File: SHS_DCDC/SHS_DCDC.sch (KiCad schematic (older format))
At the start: 16 parts, among them J1 Barrel_Jack, Q1 BSS84, U1 A0Z1283

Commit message: esp32 s2 mini placed
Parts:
- C1, C2, C3, C4, C5: symbol Device:C -> SHS_DCDC:C-Device
- J1: symbol Connector:Barrel_Jack -> SHS_DCDC:Barrel_Jack-Connector
- L1: symbol Device:L -> SHS_DCDC:L-Device
- Q1: symbol Transistor_FET:BSS84 -> SHS_DCDC:BSS84-Transistor_FET
- R1, R2, R3, R4, R5, R6, R7: symbol Device:R -> SHS_DCDC:R-Device
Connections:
- net labels added: GND-power
- net labels removed: GND
- wire segments 44 -> 42
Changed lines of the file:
@@
 $EndDescr
 $Comp
-L Device:R R1
+L SHS_DCDC:R-Device R1
 U 1 1 603C1DE3
 P 3450 1300
@@
 EN
 $Comp
-L power:GND #PWR0101
+L SHS_DCDC:GND-power #PWR0101
 U 1 1 603DA7E8
 P 4700 2100
 F 0 "#PWR0101" H 4700 1850 50  0001 C CNN
-F 1 "GND" H 4705 1927 50  0000 C CNN
+F 1 "GND-power" H 4705 1927 50  0000 C CNN
 F 2 "" H 4700 2100 50  0001 C CNN
 F 3 "" H 4700 2100 50  0001 C CNN
@@
 	4700 2100 4700 1800
 $Comp
-L Device:C C1
+L SHS_DCDC:C-Device C1
 U 1 1 603DBEB8
 P 5750 1150
@@
 	5150 1150 5600 1150
 $Comp
-L power:GND #PWR0102
+L SHS_DCDC:GND-power #PWR0102
 U 1 1 603DC622
 P 6100 1150
 F 0 "#PWR0102" H 6100 900 50  0001 C CNN
-F 1 "GND" V 6105 1022 50  0000 R CNN
+F 1 "GND-power" V 6105 1022 50  0000 R CNN
 F 2 "" H 6100 1150 50  0001 C CNN
 F 3 "" H 6100 1150 50  0001 C CNN
@@
 	6050 1850 6350 1850
 $Comp
-L Device:C C2
+L SHS_DCDC:C-Device C2
 U 1 1 603EC5C6
 P 6050 1600
@@
 $EndComp
 $Comp
-L Device:L L1
+L SHS_DCDC:L-Device L1
 U 1 1 603ED963
 P 6500 1850
@@
 	6850 3000 6850 3150
 $Comp
-L Device:R R2
+L SHS_DCDC:R-Device R2
 U 1 1 603C2934
 P 3850 1650
@@
 $EndComp
 $Comp
-L Device:R R3
+L SHS_DCDC:R-Device R3
 U 1 1 603EF351
 P 6850 2150
@@
 $EndComp
 $Comp
-L Device:R R4
+L SHS_DCDC:R-Device R4
 U 1 1 603EF915
 P 6850 3300
@@
 	6850 3450 6850 3750
 $Comp
-L power:GND #PWR02
+L SHS_DCDC:GND-power #PWR02
 U 1 1 603F0D28
 P 6850 3750
 F 0 "#PWR02" H 6850 3500 50  0001 C CNN
-F 1 "GND" H 6855 3577 50  0000 C CNN
+F 1 "GND-power" H 6855 3577 50  0000 C CNN
 F 2 "" H 6850 3750 50  0001 C CNN
 F 3 "" H 6850 3750 50  0001 C CNN
@@
 	3850 1800 3850 2250
 $Comp
-L Device:C C3
+L SHS_DCDC:C-Device C3
 U 1 1 603F1B39
 P 4100 2100
@@
 $EndComp
 $Comp
-L Device:R R5
+L SHS_DCDC:R-Device R5
 U 1 1 603F2000
 P 4100 2700
@@
 	4100 2850 4100 3250
 $Comp
-L power:GND #PWR01
+L SHS_DCDC:GND-power #PWR01
 U 1 1 603F2C50
 P 4100 3250
 F 0 "#PWR01" H 4100 3000 50  0001 C CNN
-F 1 "GND" H 4105 3077 50  0000 C CNN
+F 1 "GND-power" H 4105 3077 50  0000 C CNN
 F 2 "" H 4100 3250 50  0001 C CNN
 F 3 "" H 4100 3250 50  0001 C CNN
@@
 	1    0    0    -1
 $EndComp
-Wire Wire Line
-	3300 1300 3050 1300
-Wire Wire Line
-	3050 1300 3050 1650
-$Comp
-L power:GND #PWR0103
+$Comp
+L SHS_DCDC:GND-power #PWR0103
 U 1 1 603FB2AC
-P 3050 1650
-F 0 "#PWR0103" H 3050 1400 50  0001 C CNN
-F 1 "GND" H 3055 1477 50  0000 C CNN
-F 2 "" H 3050 1650 50  0001 C CNN
-F 3 "" H 3050 1650 50  0001 C CNN
-	1    3050 1650
-	1    0    0    -1
-$EndComp
-$Comp
-L Transistor_FET:BSS84 Q1
+P 3000 1300
+F 0 "#PWR0103" H 3000 1050 50  0001 C CNN
+F 1 "GND-power" H 3005 1127 50  0000 C CNN
+F 2 "" H 3000 1300 50  0001 C CNN
+F 3 "" H 3000 1300 50  0001 C CNN
+	1    3000 1300
+	0    1    1    0
+$EndComp
+$Comp
+L SHS_DCDC:BSS84-Transistor_FET Q1
 U 1 1 60436C74
 P 6950 2700
@@
 	7150 2700 7650 2700
 $Comp
-L Device:C C4
+L SHS_DCDC:C-Device C4
 U 1 1 604424F8
 P 7650 3000
@@
 $EndComp
 $Comp
-L Device:C C5
+L SHS_DCDC:C-Device C5
 U 1 1 60442BC9
 P 8100 3000
@@
 Connection ~ 8100 2700
 $Comp
-L Device:R R6
+L SHS_DCDC:R-Device R6
 U 1 1 6044493A
 P 8550 2700
@@
 	9100 2700 9100 2850
 $Comp
-L Device:R R7
+L SHS_DCDC:R-Device R7
 U 1 1 60446ABA
 P 9100 3000
@@
 Connection ~ 9100 2700
 $Comp
-L power:GND #PWR03
+L SHS_DCDC:GND-power #PWR03
 U 1 1 60449010
 P 7650 3350
 F 0 "#PWR03" H 7650 3100 50  0001 C CNN
-F 1 "GND" H 7655 3177 50  0000 C CNN
+F 1 "GND-power" H 7655 3177 50  0000 C CNN
 F 2 "" H 7650 3350 50  0001 C CNN
 F 3 "" H 7650 3350 50  0001 C CNN
@@
 $EndComp
 $Comp
-L power:GND #PWR04
+L SHS_DCDC:GND-power #PWR04
 U 1 1 60449366
 P 8100 3350
 F 0 "#PWR04" H 8100 3100 50  0001 C CNN
-F 1 "GND" H 8105 3177 50  0000 C CNN
+F 1 "GND-power" H 8105 3177 50  0000 C CNN
 F 2 "" H 8100 3350 50  0001 C CNN
 F 3 "" H 8100 3350 50  0001 C CNN
@@
 $EndComp
 $Comp
-L power:GND #PWR05
+L SHS_DCDC:GND-power #PWR05
 U 1 1 60449544
 P 9100 3350
 F 0 "#PWR05" H 9100 3100 50  0001 C CNN
-F 1 "GND" H 9105 3177 50  0000 C CNN
+F 1 "GND-power" H 9105 3177 50  0000 C CNN
 F 2 "" H 9100 3350 50  0001 C CNN
 F 3 "" H 9100 3350 50  0001 C CNN
@@
 $EndSheet
 $Comp
-L Connector:Barrel_Jack J1
+L SHS_DCDC:Barrel_Jack-Connector J1
 U 1 1 604EA25D
 P 2100 1250
@@
 	1    0    0    -1
 $EndComp
-Wire Wire Line
-	2400 1350 2700 1350
-Wire Wire Line
-	2700 1350 2700 1650
-$Comp
-L power:GND #PWR0104
+$Comp
+L SHS_DCDC:GND-power #PWR0104
 U 1 1 604EC198
-P 2700 1650
-F 0 "#PWR0104" H 2700 1400 50  0001 C CNN
-F 1 "GND" H 2705 1477 50  0000 C CNN
-F 2 "" H 2700 1650 50  0001 C CNN
-F 3 "" H 2700 1650 50  0001 C CNN
-	1    2700 1650
-	1    0    0    -1
+P 2550 1350
+F 0 "#PWR0104" H 2550 1100 50  0001 C CNN
+F 1 "GND-power" H 2555 1177 50  0000 C CNN
+F 2 "" H 2550 1350 50  0001 C CNN
+F 3 "" H 2550 1350 50  0001 C CNN
+	1    2550 1350
+	0    -1   -1   0
 $EndComp
 $Sheet
@@
 F1 "USB.sch" 50
 $EndSheet
+Wire Wire Line
+	3000 1300 3300 1300
+Wire Wire Line
+	2400 1350 2550 1350
 $EndSCHEMATC

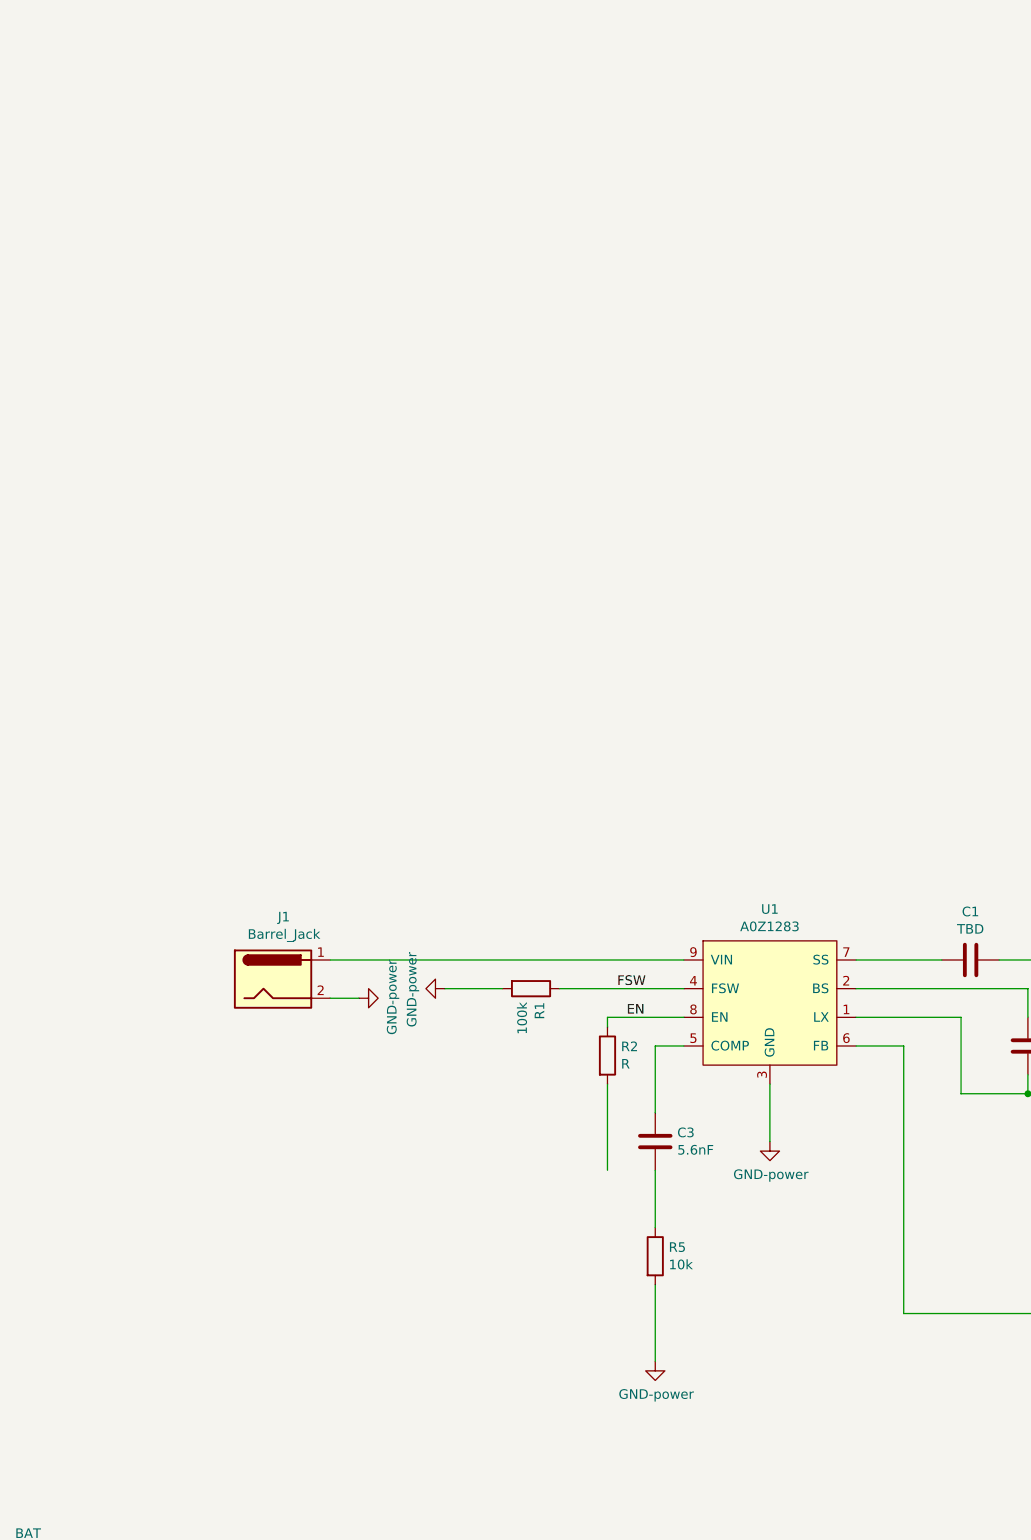
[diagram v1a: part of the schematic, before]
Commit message: Commit_GitHubgDesktop
Try of Github desktop
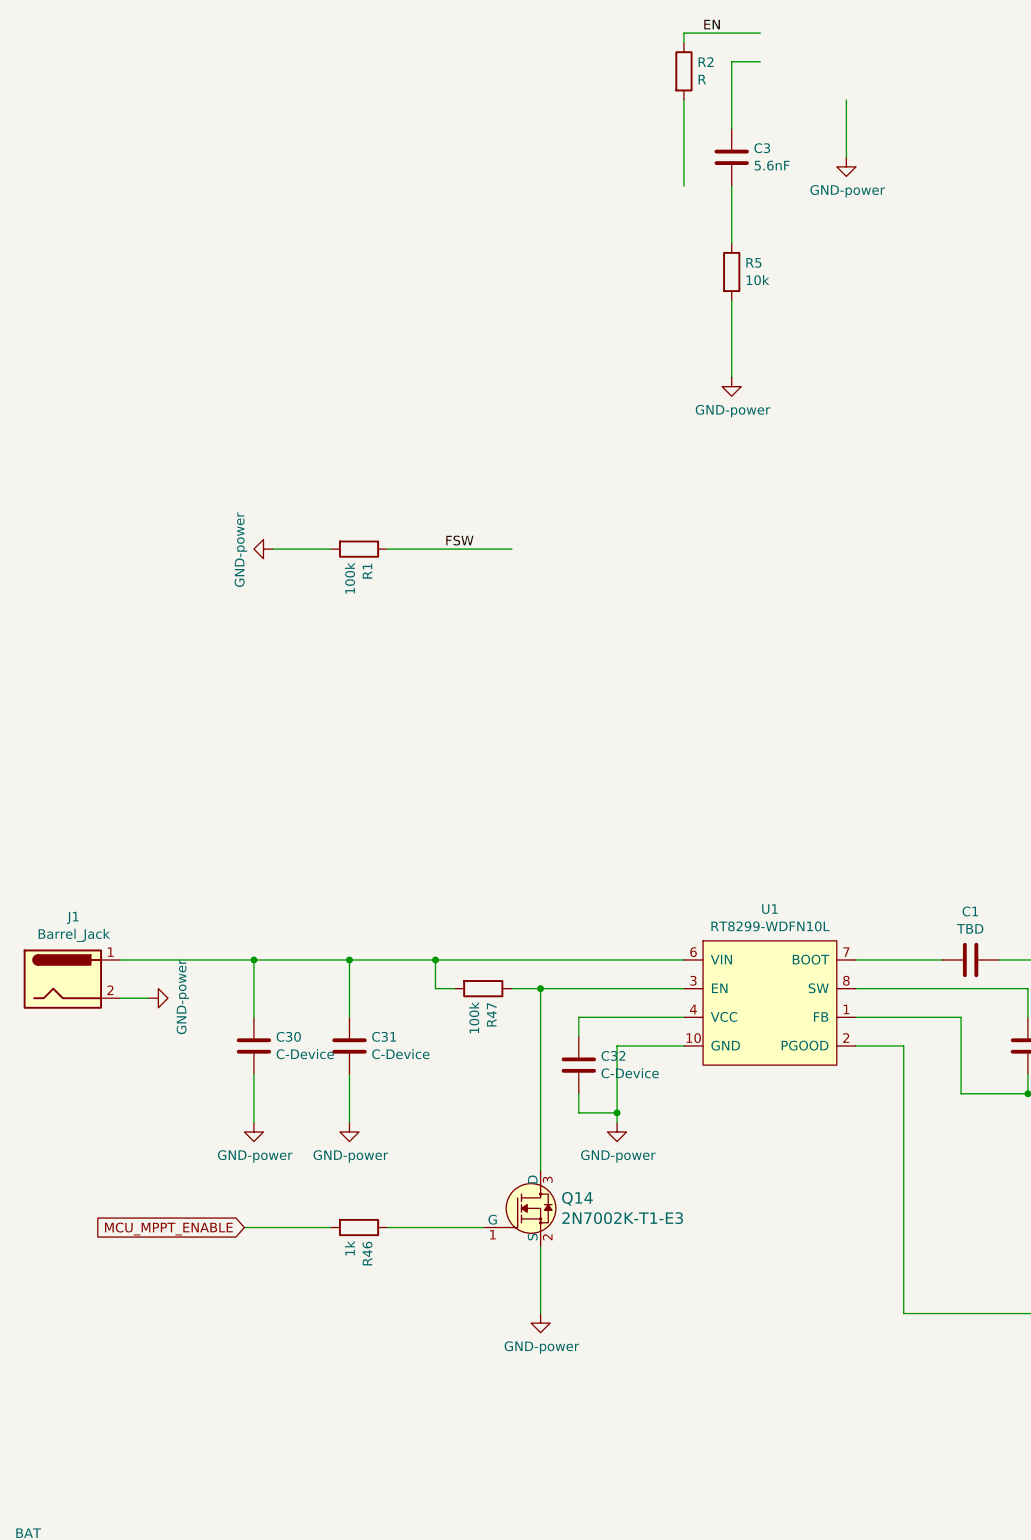
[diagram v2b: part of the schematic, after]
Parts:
- removed U1: A0Z1283, SHS_DCDC:SOIC-8, symbol SHS_DCDC:A0Z1283
- added C30, C31, C32: C-Device, symbol SHS_DCDC:C-Device
- added Q14: 2N7002K-T1-E3, digikey-footprints:SOT-23-3, symbol dk_Transistors-FETs-MOSFETs-Single:2N7002K-T1-E3
- added R46: 1k, Resistor_SMD:R_0603_1608Metric, symbol SHS_DCDC:R-Device
- added R47: 100k, Resistor_SMD:R_0603_1608Metric, symbol SHS_DCDC:R-Device
- added U1: RT8299-WDFN10L, symbol SHS_DCDC:RT8299-WDFN10L
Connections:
- net labels added: MCU_MPPT_ENABLE
- wire segments 42 -> 64
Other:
- moved on the sheet: C3, J1, R1, R2, R5
